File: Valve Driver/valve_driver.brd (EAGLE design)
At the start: 80 x 80 mm, 15 parts

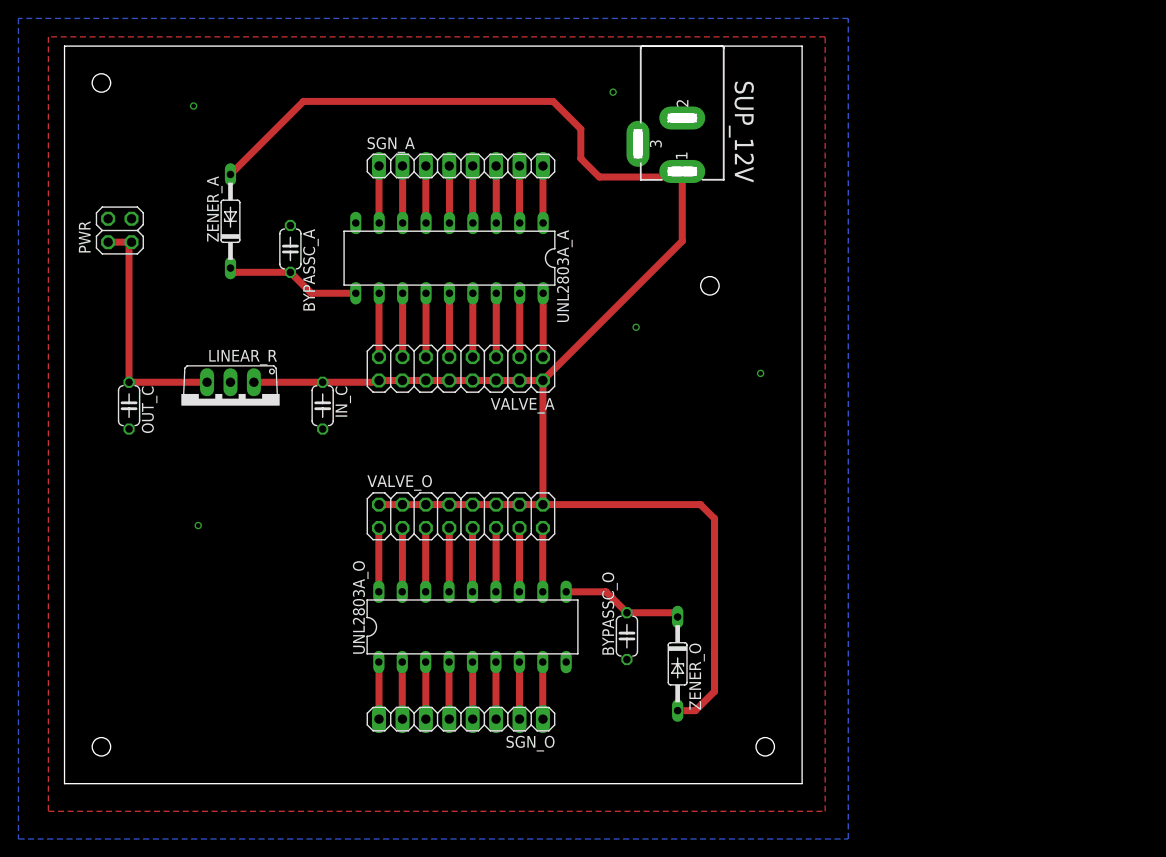
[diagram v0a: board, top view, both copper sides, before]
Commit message: Revert "20180712-change-pin"
This reverts commit fb38f18733497d936434fddb3c409504ab7d6048.
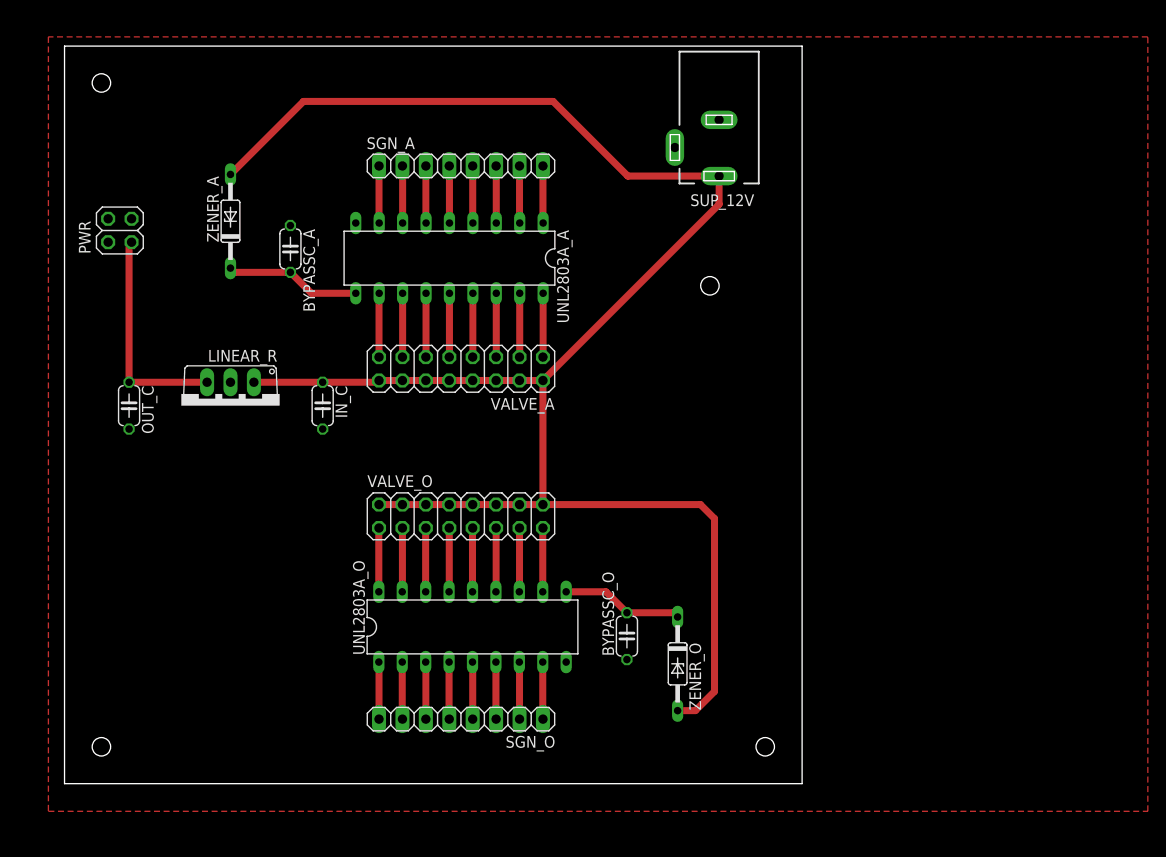
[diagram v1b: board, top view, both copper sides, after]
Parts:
- SUP_12V: value (none) -> DCJ0202; device mylib:69410X301002 -> con-jack:DCJ0202
- moved SUP_12V 11.7 mm to (71.0, 69.0), turned to 180 degrees
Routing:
- net VCCH: track 192.2 -> 195.2 mm
- net VCCL: track 26.3 -> 23.8 mm
- removed copper zone on layer 16, net GND
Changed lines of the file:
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@@
 <setting verticaltext="up"/>
 </settings>
-<grid distance="0.1" unitdist="mm" unit="mm" style="lines" multiple="1" display="yes" altdistance="1" altunitdist="mm" altunit="mm"/>
+<grid distance="1" unitdist="mm" unit="mm" style="lines" multiple="1" display="yes" altdistance="1" altunitdist="mm" altunit="mm"/>
 <layers>
 <layer number="1" name="Top" color="4" fill="1" visible="yes" active="yes"/>
@@
 <layer number="42" name="bRestrict" color="1" fill="10" visible="no" active="yes"/>
 <layer number="43" name="vRestrict" color="2" fill="10" visible="no" active="yes"/>
-<layer number="44" name="Drills" color="7" fill="1" visible="yes" active="yes"/>
+<layer number="44" name="Drills" color="7" fill="1" visible="no" active="yes"/>
 <layer number="45" name="Holes" color="7" fill="1" visible="yes" active="yes"/>
 <layer number="46" name="Milling" color="3" fill="1" visible="no" active="yes"/>
@@
 <layer number="228" name="228bmp" color="7" fill="1" visible="yes" active="yes"/>
 <layer number="229" name="229bmp" color="7" fill="1" visible="yes" active="yes"/>
-<layer number="230" name="230bmp" color="7" fill="1" visible="no" active="yes"/>
+<layer number="230" name="230bmp" color="7" fill="1" visible="yes" active="yes"/>
 <layer number="231" name="Eagle3D_PG1" color="7" fill="1" visible="no" active="no"/>
 <layer number="232" name="Eagle3D_PG2" color="7" fill="1" visible="no" active="no"/>
@@
 <attribute name="OC_NEWARK" value="unknown" x="66.5" y="13" size="1.778" layer="27" rot="R270" display="off"/>
 </element>
-<element name="SUP_12V" library="mylib" package="69410X301002" package3d_urn="urn:adsk.eagle:package:3359594/1" value="" x="67" y="80" rot="R270"/>
+<element name="SUP_12V" library="con-jack" library_urn="urn:adsk.eagle:library:154" package="DCJ0202" package3d_urn="urn:adsk.eagle:package:7491/1" value="DCJ0202" x="71" y="69" rot="R180">
+<attribute name="MF" value="" x="96" y="42.75" size="1.778" layer="27" rot="R180" display="off"/>
+<attribute name="MPN" value="" x="96" y="42.75" size="1.778" layer="27" rot="R180" display="off"/>
+<attribute name="OC_FARNELL" value="unknown" x="96" y="42.75" size="1.778" layer="27" rot="R180" display="off"/>
+<attribute name="OC_NEWARK" value="unknown" x="96" y="42.75" size="1.778" layer="27" rot="R180" display="off"/>
+</element>
 <element name="VALVE_A" library="pinhead" library_urn="urn:adsk.eagle:library:325" package="2X08" package3d_urn="urn:adsk.eagle:package:22481/2" value="" x="43" y="45" rot="R180"/>
 <element name="VALVE_O" library="pinhead" library_urn="urn:adsk.eagle:library:325" package="2X08" package3d_urn="urn:adsk.eagle:package:22481/2" value="" x="43" y="29"/>
@@
 <vertex x="-1.75" y="81"/>
 <vertex x="-1.75" y="-3"/>
-<vertex x="82.5" y="-3"/>
-<vertex x="82.5" y="81"/>
+<vertex x="117.5" y="-3"/>
+<vertex x="117.5" y="81"/>
 </polygon>
-<polygon width="0.762" layer="16">
-<vertex x="-5" y="83"/>
-<vertex x="-5" y="-6"/>
-<vertex x="85" y="-6"/>
-<vertex x="85" y="83"/>
-</polygon>
-<via x="75.5" y="44.5" extent="1-16" drill="0.508"/>
-<via x="59.5" y="75" extent="1-16" drill="0.508"/>
-<via x="62" y="49.5" extent="1-16" drill="0.508"/>
-<via x="14.5" y="28" extent="1-16" drill="0.508"/>
-<via x="14" y="73.5" extent="1-16" drill="0.508"/>
 </signal>
 <signal name="VCCL">
@@
 <wire x1="7" y1="43.54" x2="7" y2="58.46" width="0.762" layer="1"/>
 <wire x1="7" y1="58.46" x2="7.27" y2="58.73" width="0.762" layer="1"/>
-<wire x1="4.73" y1="58.73" x2="7.27" y2="58.73" width="0.762" layer="1"/>
+<wire x1="7" y1="58.46" x2="4.73" y2="58.73" width="0" layer="19" extent="1-1"/>
 </signal>
 <signal name="COM2">
@@
 <wire x1="28" y1="43.54" x2="20.54" y2="43.54" width="0.762" layer="1"/>
 <wire x1="18" y1="66.08" x2="25.92" y2="74" width="0.762" layer="1"/>
+<wire x1="61.1" y1="65.9" x2="71" y2="65.9" width="0.762" layer="1"/>
 <wire x1="25.92" y1="74" x2="53" y2="74" width="0.762" layer="1"/>
-<wire x1="51.89" y1="43.73" x2="67" y2="58.84" width="0.762" layer="1"/>
-<wire x1="67" y1="58.84" x2="67" y2="66.4" width="0.762" layer="1"/>
-<wire x1="53" y1="74" x2="56" y2="71" width="0.762" layer="1"/>
-<wire x1="56" y1="67.8" x2="58" y2="65.8" width="0.762" layer="1"/>
-<wire x1="58" y1="65.8" x2="66.4" y2="65.8" width="0.762" layer="1"/>
-<wire x1="66.4" y1="65.8" x2="67" y2="66.4" width="0.762" layer="1"/>
-<wire x1="56" y1="71" x2="56" y2="67.8" width="0.762" layer="1"/>
+<wire x1="53" y1="74" x2="61.1" y2="65.9" width="0.762" layer="1"/>
+<wire x1="71" y1="65.9" x2="71" y2="62.84" width="0.762" layer="1"/>
+<wire x1="71" y1="62.84" x2="51.89" y2="43.73" width="0.762" layer="1"/>
 </signal>
 <signal name="N$1">

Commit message: 20180712-change-pin
change ch1's pin to right(10):
right(11,12) is not avaliable
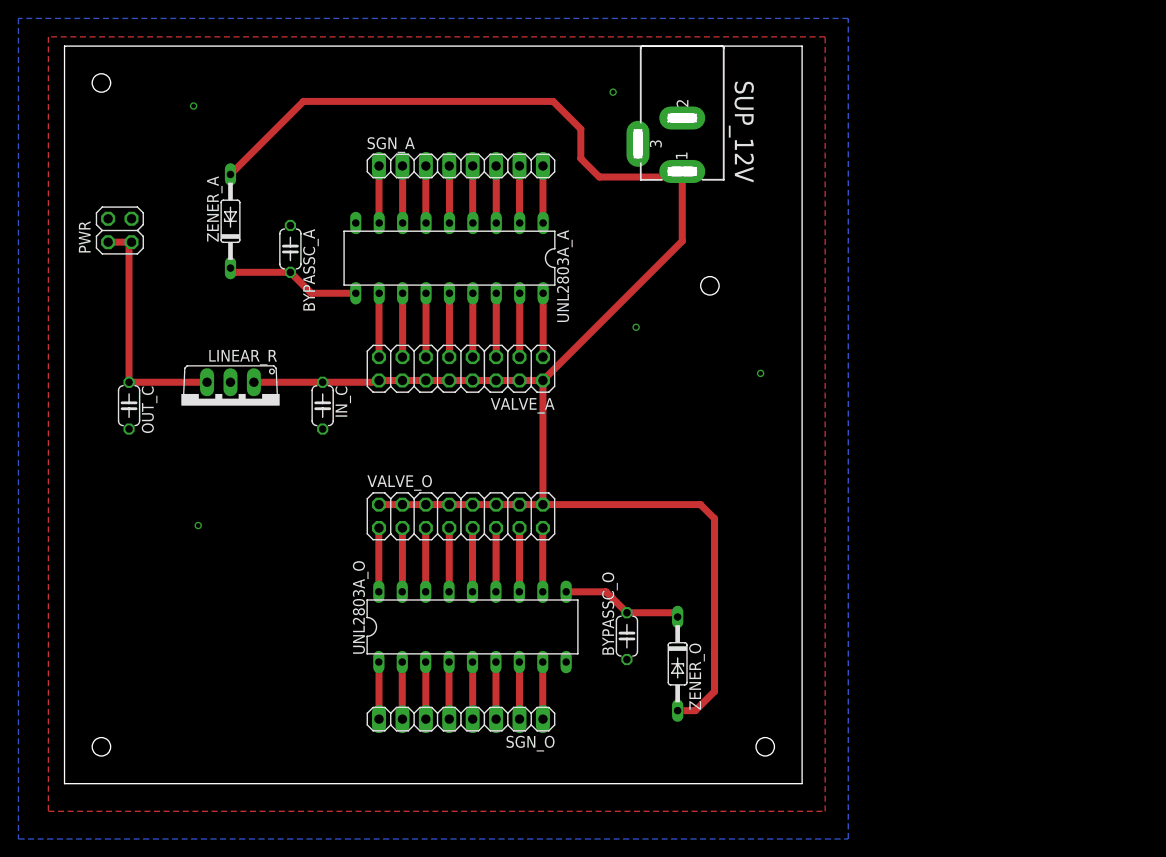
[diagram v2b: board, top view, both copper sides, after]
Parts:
- SUP_12V: value DCJ0202 -> (none); device con-jack:DCJ0202 -> mylib:69410X301002
- moved SUP_12V 11.7 mm to (67.0, 80.0), turned to 270 degrees
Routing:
- net VCCH: track 195.2 -> 192.2 mm
- net VCCL: track 23.8 -> 26.3 mm
- added copper zone on layer 16, net GND
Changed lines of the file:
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@@
 <setting verticaltext="up"/>
 </settings>
-<grid distance="1" unitdist="mm" unit="mm" style="lines" multiple="1" display="yes" altdistance="1" altunitdist="mm" altunit="mm"/>
+<grid distance="0.1" unitdist="mm" unit="mm" style="lines" multiple="1" display="yes" altdistance="1" altunitdist="mm" altunit="mm"/>
 <layers>
 <layer number="1" name="Top" color="4" fill="1" visible="yes" active="yes"/>
@@
 <layer number="42" name="bRestrict" color="1" fill="10" visible="no" active="yes"/>
 <layer number="43" name="vRestrict" color="2" fill="10" visible="no" active="yes"/>
-<layer number="44" name="Drills" color="7" fill="1" visible="no" active="yes"/>
+<layer number="44" name="Drills" color="7" fill="1" visible="yes" active="yes"/>
 <layer number="45" name="Holes" color="7" fill="1" visible="yes" active="yes"/>
 <layer number="46" name="Milling" color="3" fill="1" visible="no" active="yes"/>
@@
 <layer number="228" name="228bmp" color="7" fill="1" visible="yes" active="yes"/>
 <layer number="229" name="229bmp" color="7" fill="1" visible="yes" active="yes"/>
-<layer number="230" name="230bmp" color="7" fill="1" visible="yes" active="yes"/>
+<layer number="230" name="230bmp" color="7" fill="1" visible="no" active="yes"/>
 <layer number="231" name="Eagle3D_PG1" color="7" fill="1" visible="no" active="no"/>
 <layer number="232" name="Eagle3D_PG2" color="7" fill="1" visible="no" active="no"/>
@@
 <attribute name="OC_NEWARK" value="unknown" x="66.5" y="13" size="1.778" layer="27" rot="R270" display="off"/>
 </element>
-<element name="SUP_12V" library="con-jack" library_urn="urn:adsk.eagle:library:154" package="DCJ0202" package3d_urn="urn:adsk.eagle:package:7491/1" value="DCJ0202" x="71" y="69" rot="R180">
-<attribute name="MF" value="" x="96" y="42.75" size="1.778" layer="27" rot="R180" display="off"/>
-<attribute name="MPN" value="" x="96" y="42.75" size="1.778" layer="27" rot="R180" display="off"/>
-<attribute name="OC_FARNELL" value="unknown" x="96" y="42.75" size="1.778" layer="27" rot="R180" display="off"/>
-<attribute name="OC_NEWARK" value="unknown" x="96" y="42.75" size="1.778" layer="27" rot="R180" display="off"/>
-</element>
+<element name="SUP_12V" library="mylib" package="69410X301002" package3d_urn="urn:adsk.eagle:package:3359594/1" value="" x="67" y="80" rot="R270"/>
 <element name="VALVE_A" library="pinhead" library_urn="urn:adsk.eagle:library:325" package="2X08" package3d_urn="urn:adsk.eagle:package:22481/2" value="" x="43" y="45" rot="R180"/>
 <element name="VALVE_O" library="pinhead" library_urn="urn:adsk.eagle:library:325" package="2X08" package3d_urn="urn:adsk.eagle:package:22481/2" value="" x="43" y="29"/>
@@
 <vertex x="-1.75" y="81"/>
 <vertex x="-1.75" y="-3"/>
-<vertex x="117.5" y="-3"/>
-<vertex x="117.5" y="81"/>
+<vertex x="82.5" y="-3"/>
+<vertex x="82.5" y="81"/>
 </polygon>
+<polygon width="0.762" layer="16">
+<vertex x="-5" y="83"/>
+<vertex x="-5" y="-6"/>
+<vertex x="85" y="-6"/>
+<vertex x="85" y="83"/>
+</polygon>
+<via x="75.5" y="44.5" extent="1-16" drill="0.508"/>
+<via x="59.5" y="75" extent="1-16" drill="0.508"/>
+<via x="62" y="49.5" extent="1-16" drill="0.508"/>
+<via x="14.5" y="28" extent="1-16" drill="0.508"/>
+<via x="14" y="73.5" extent="1-16" drill="0.508"/>
 </signal>
 <signal name="VCCL">
@@
 <wire x1="7" y1="43.54" x2="7" y2="58.46" width="0.762" layer="1"/>
 <wire x1="7" y1="58.46" x2="7.27" y2="58.73" width="0.762" layer="1"/>
-<wire x1="7" y1="58.46" x2="4.73" y2="58.73" width="0" layer="19" extent="1-1"/>
+<wire x1="4.73" y1="58.73" x2="7.27" y2="58.73" width="0.762" layer="1"/>
 </signal>
 <signal name="COM2">
@@
 <wire x1="28" y1="43.54" x2="20.54" y2="43.54" width="0.762" layer="1"/>
 <wire x1="18" y1="66.08" x2="25.92" y2="74" width="0.762" layer="1"/>
-<wire x1="61.1" y1="65.9" x2="71" y2="65.9" width="0.762" layer="1"/>
 <wire x1="25.92" y1="74" x2="53" y2="74" width="0.762" layer="1"/>
-<wire x1="53" y1="74" x2="61.1" y2="65.9" width="0.762" layer="1"/>
-<wire x1="71" y1="65.9" x2="71" y2="62.84" width="0.762" layer="1"/>
-<wire x1="71" y1="62.84" x2="51.89" y2="43.73" width="0.762" layer="1"/>
+<wire x1="51.89" y1="43.73" x2="67" y2="58.84" width="0.762" layer="1"/>
+<wire x1="67" y1="58.84" x2="67" y2="66.4" width="0.762" layer="1"/>
+<wire x1="53" y1="74" x2="56" y2="71" width="0.762" layer="1"/>
+<wire x1="56" y1="67.8" x2="58" y2="65.8" width="0.762" layer="1"/>
+<wire x1="58" y1="65.8" x2="66.4" y2="65.8" width="0.762" layer="1"/>
+<wire x1="66.4" y1="65.8" x2="67" y2="66.4" width="0.762" layer="1"/>
+<wire x1="56" y1="71" x2="56" y2="67.8" width="0.762" layer="1"/>
 </signal>
 <signal name="N$1">
